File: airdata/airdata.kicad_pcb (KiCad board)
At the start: 2 copper layers, 37.8 x 6 mm, 19 parts, among them J1 I2C, J2 I2C, U1 SDP32, U2 MS5611-01BA03, U3 SDP32, U4 LT1761-3.3, U5 HSCMRRN001PD2A3, U6 SDP32

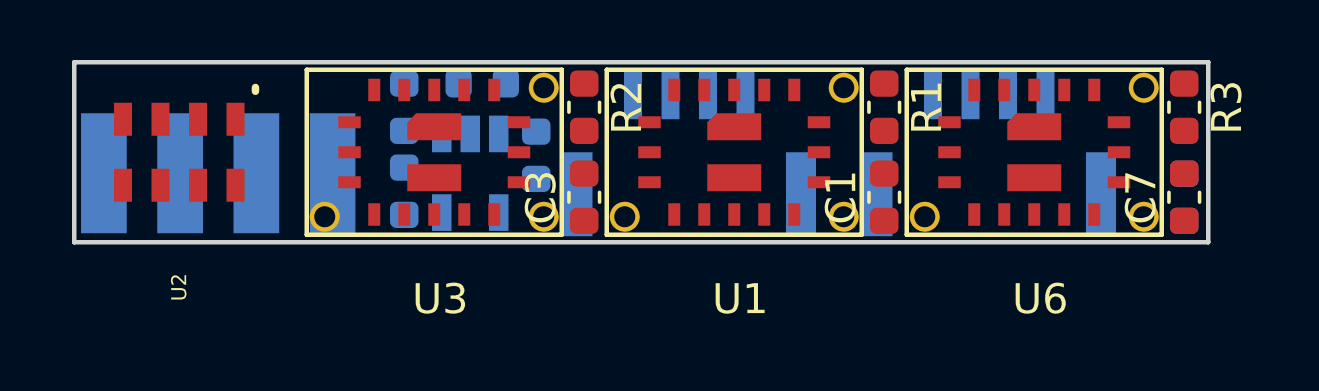
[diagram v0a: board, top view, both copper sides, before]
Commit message: airdata & power supply pcb
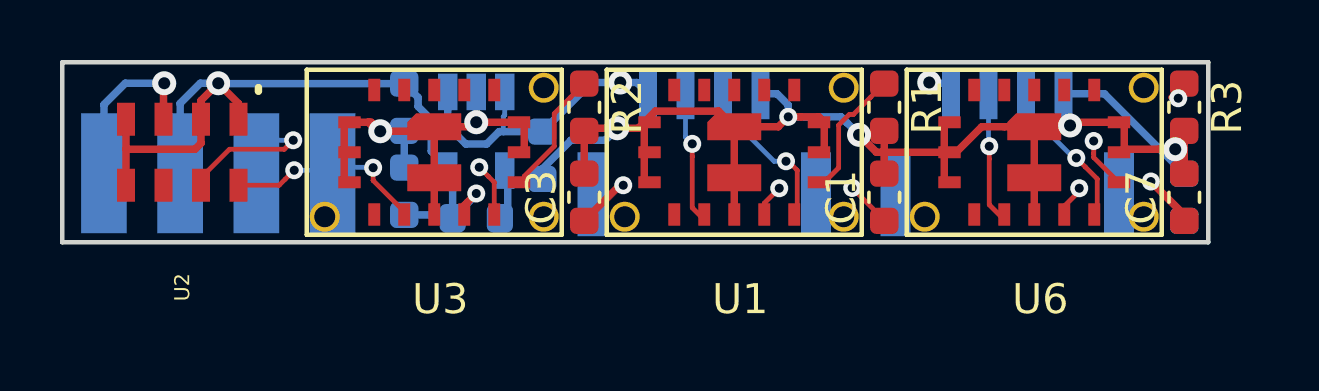
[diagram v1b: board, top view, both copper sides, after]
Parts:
- moved C4 3.12 mm to (43.6, 32.6), turned to 270 degrees
- moved C6 2.90 mm to (41.4, 34.7), turned to 0 degrees
- moved U4 1.41 mm to (41.4, 31.8)
- moved J1 0.60 mm to (59.1, 32.5)
- moved J2 0.50 mm to (49.0, 32.5)
- moved U2 0.10 mm to (31.6, 32.5)
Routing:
- net GND: track 0.00 -> 111.3 mm, vias 0 -> 8
- net +3V3: track 0.00 -> 70.6 mm, vias 0 -> 7
- net /SDA: track 0.00 -> 47.0 mm, vias 0 -> 4
- net /SCL: track 0.00 -> 37.0 mm, vias 0 -> 4
- net +5V: track 0.00 -> 33.9 mm, vias 0 -> 2
- net Net-(R3-Pad1): track 0.00 -> 6.54 mm, vias 0 -> 2
- net Net-(R1-Pad1): track 0.00 -> 4.20 mm
- net Net-(R2-Pad1): track 0.00 -> 4.12 mm
- net Net-(C6-Pad2): track 0.00 -> 1.70 mm
- added copper zone on In1.Cu, net GND
- added copper zone on In2.Cu, net GND
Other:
- board size 37.8 x 6 mm -> 38.2 x 6 mm
- copper layers 2 -> 4
- rule trace_min: 0.2 -> 0.152
- rule via_min_size: 0.4 -> 0.6
